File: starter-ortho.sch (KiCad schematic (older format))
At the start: 98 parts, among them SW1 SW_Push, U1 ProMicro

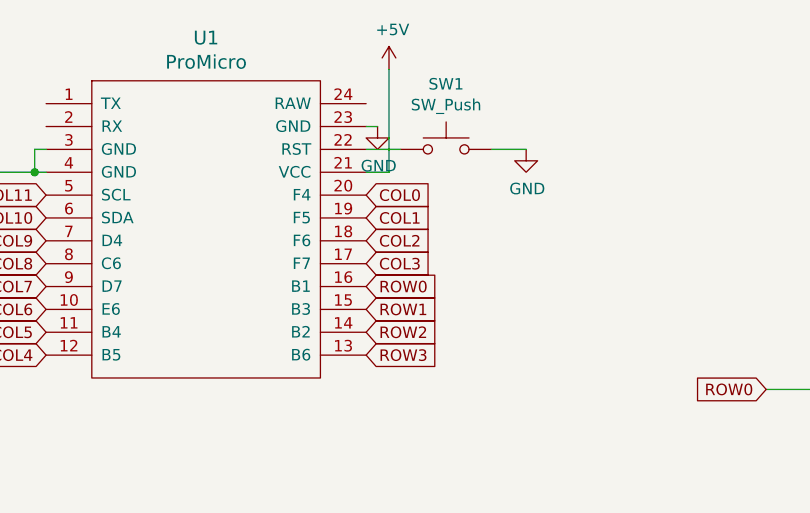
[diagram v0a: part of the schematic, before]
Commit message: Routed traces (poorly)
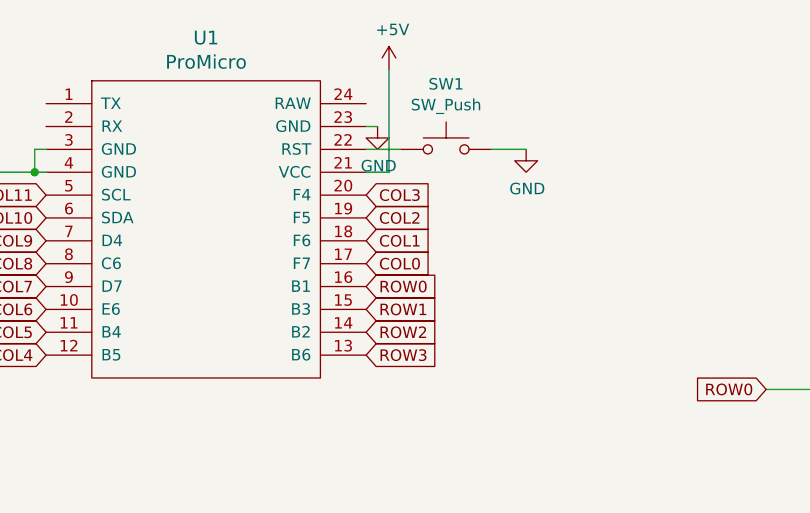
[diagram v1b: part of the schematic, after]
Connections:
- net COL0: now also U1.17 (F7); no longer U1.20 (F4)
- net COL1: now also U1.18 (F6); no longer U1.19 (F5)
- net COL2: now also U1.19 (F5); no longer U1.18 (F6)
- net COL3: now also U1.20 (F4); no longer U1.17 (F7)
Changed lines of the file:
@@
 Wire Wire Line
 	3600 2100 3750 2100
-Text GLabel 3050 2700 2    50   Input ~ 0
-ROW0
-Text GLabel 3050 2800 2    50   Input ~ 0
-ROW1
-Text GLabel 3050 2900 2    50   Input ~ 0
-ROW2
-Text GLabel 3050 3000 2    50   Input ~ 0
-ROW3
-Text GLabel 3050 2300 2    50   Input ~ 0
-COL0
-Text GLabel 3050 2400 2    50   Input ~ 0
-COL1
-Text GLabel 3050 2500 2    50   Input ~ 0
-COL2
-Text GLabel 3050 2600 2    50   Input ~ 0
-COL3
 Text GLabel 1650 3000 0    50   Input ~ 0
 COL4
@@
 Wire Wire Line
 	1600 2200 1250 2200
+Text GLabel 3050 3000 2    50   Input ~ 0
+ROW3
+Text GLabel 3050 2900 2    50   Input ~ 0
+ROW2
+Text GLabel 3050 2800 2    50   Input ~ 0
+ROW1
+Text GLabel 3050 2700 2    50   Input ~ 0
+ROW0
+Text GLabel 3050 2400 2    50   Input ~ 0
+COL2
+Text GLabel 3050 2600 2    50   Input ~ 0
+COL0
+Text GLabel 3050 2500 2    50   Input ~ 0
+COL1
+Text GLabel 3050 2300 2    50   Input ~ 0
+COL3
 $EndSCHEMATC

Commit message: we're doing choc switches now baby
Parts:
- MX1, MX10, MX11, MX12, MX13, MX14, MX15, MX16, MX17, MX18, MX19, MX2, MX20, MX21, MX22, MX23, MX24, MX25, MX26, MX27, MX28, MX29, MX3, MX30, MX31, MX32, MX33, MX34, MX35, MX36, MX37, MX38, MX39, MX4, MX40, MX41, MX42, MX43, MX44, MX45, MX46, MX47, MX48, MX5, MX6, MX7, MX8, MX9: footprint MX_Alps_Hybrid:MX-1U-NoLED -> Kailh_Choc:KailhChoc-1U

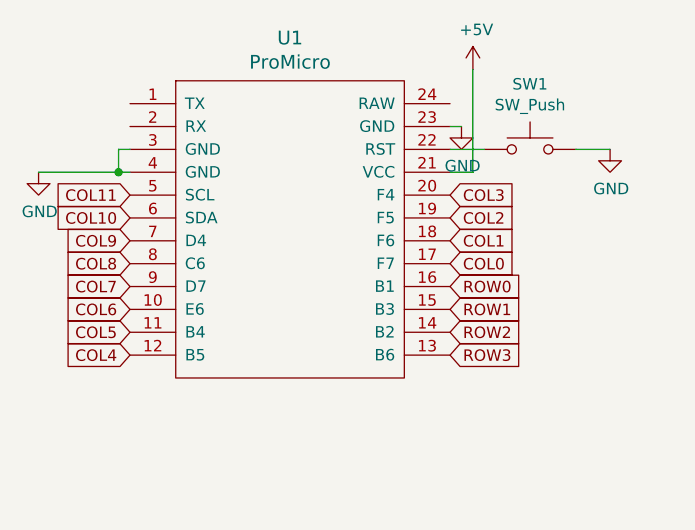
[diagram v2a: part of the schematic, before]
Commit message: all traces routed
done well? we'll see...
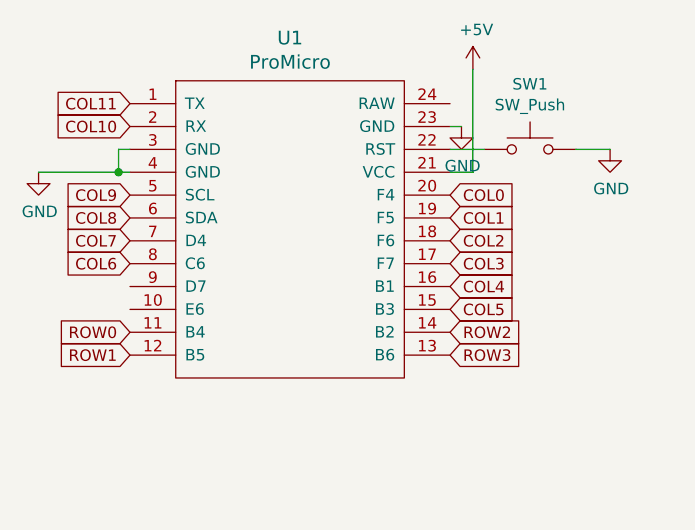
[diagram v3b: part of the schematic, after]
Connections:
- net COL0: now also U1.20 (F4); no longer U1.17 (F7)
- net COL1: now also U1.19 (F5); no longer U1.18 (F6)
- net COL10: now also U1.2 (RX); no longer U1.6 (SDA)
- net COL11: now also U1.1 (TX); no longer U1.5 (SCL)
- net COL2: now also U1.18 (F6); no longer U1.19 (F5)
- net COL3: now also U1.17 (F7); no longer U1.20 (F4)
- net COL4: now also U1.16 (B1); no longer U1.12 (B5)
- net COL5: now also U1.15 (B3); no longer U1.11 (B4)
- net COL6: now also U1.8 (C6); no longer U1.10 (E6)
- net COL7: now also U1.7 (D4); no longer U1.9 (D7)
- net COL8: now also U1.6 (SDA); no longer U1.8 (C6)
- net COL9: now also U1.5 (SCL); no longer U1.7 (D4)
- net ROW0: now also U1.11 (B4); no longer U1.16 (B1)
- net ROW1: now also U1.12 (B5); no longer U1.15 (B3)
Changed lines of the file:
@@
 Wire Wire Line
 	3600 2100 3750 2100
-Text GLabel 1650 3000 0    50   Input ~ 0
+Text GLabel 3050 2700 2    50   Input ~ 0
 COL4
-Text GLabel 1650 2900 0    50   Input ~ 0
+Text GLabel 3050 2800 2    50   Input ~ 0
 COL5
-Text GLabel 1650 2800 0    50   Input ~ 0
+Text GLabel 1650 2600 0    50   Input ~ 0
 COL6
-Text GLabel 1650 2700 0    50   Input ~ 0
+Text GLabel 1650 2500 0    50   Input ~ 0
 COL7
-Text GLabel 1650 2600 0    50   Input ~ 0
+Text GLabel 1650 2400 0    50   Input ~ 0
 COL8
-Text GLabel 1650 2500 0    50   Input ~ 0
+Text GLabel 1650 2300 0    50   Input ~ 0
 COL9
-Text GLabel 1650 2400 0    50   Input ~ 0
+Text GLabel 1650 2000 0    50   Input ~ 0
 COL10
-Text GLabel 1650 2300 0    50   Input ~ 0
+Text GLabel 1650 1900 0    50   Input ~ 0
 COL11
 $Comp
@@
 Text GLabel 3050 2900 2    50   Input ~ 0
 ROW2
-Text GLabel 3050 2800 2    50   Input ~ 0
+Text GLabel 1650 3000 0    50   Input ~ 0
 ROW1
-Text GLabel 3050 2700 2    50   Input ~ 0
+Text GLabel 1650 2900 0    50   Input ~ 0
 ROW0
+Text GLabel 3050 2500 2    50   Input ~ 0
+COL2
+Text GLabel 3050 2300 2    50   Input ~ 0
+COL0
 Text GLabel 3050 2400 2    50   Input ~ 0
-COL2
+COL1
 Text GLabel 3050 2600 2    50   Input ~ 0
-COL0
-Text GLabel 3050 2500 2    50   Input ~ 0
-COL1
-Text GLabel 3050 2300 2    50   Input ~ 0
 COL3
 $EndSCHEMATC
